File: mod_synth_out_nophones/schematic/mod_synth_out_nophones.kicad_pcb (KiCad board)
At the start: 2 copper layers, 81.9 x 109.2 mm, 50 parts, among them J1 L IN, J2 R IN, J3 Conn_02x08_Odd_Even, J5 L OUT, J6 R OUT, J7 Conn_01x07_Female, J8 Conn_01x07_Male, Q1 2N3904, Q2 2N3904, U1 TL072, U2 TL072

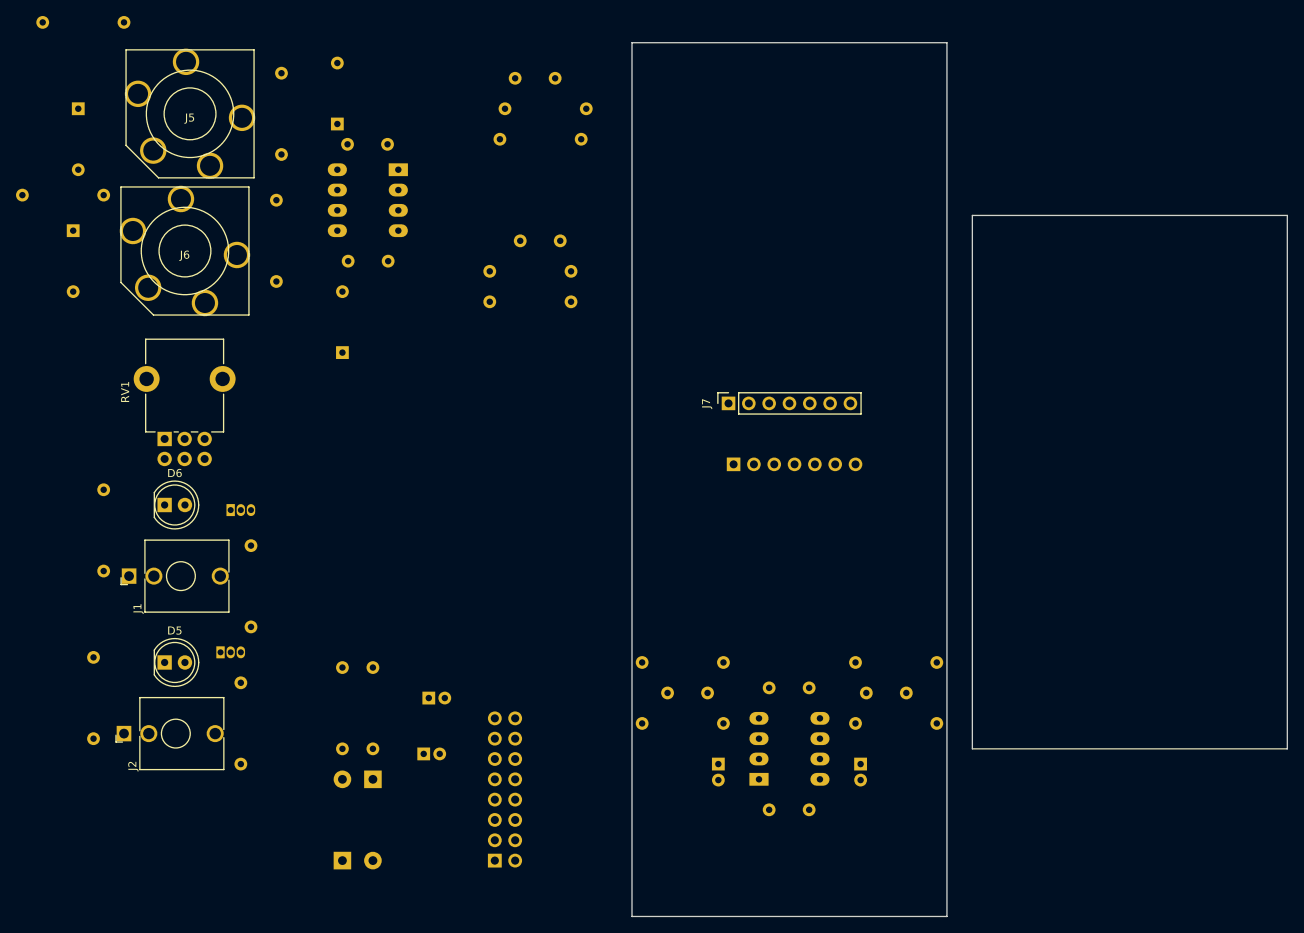
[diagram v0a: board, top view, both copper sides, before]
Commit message: Layout components
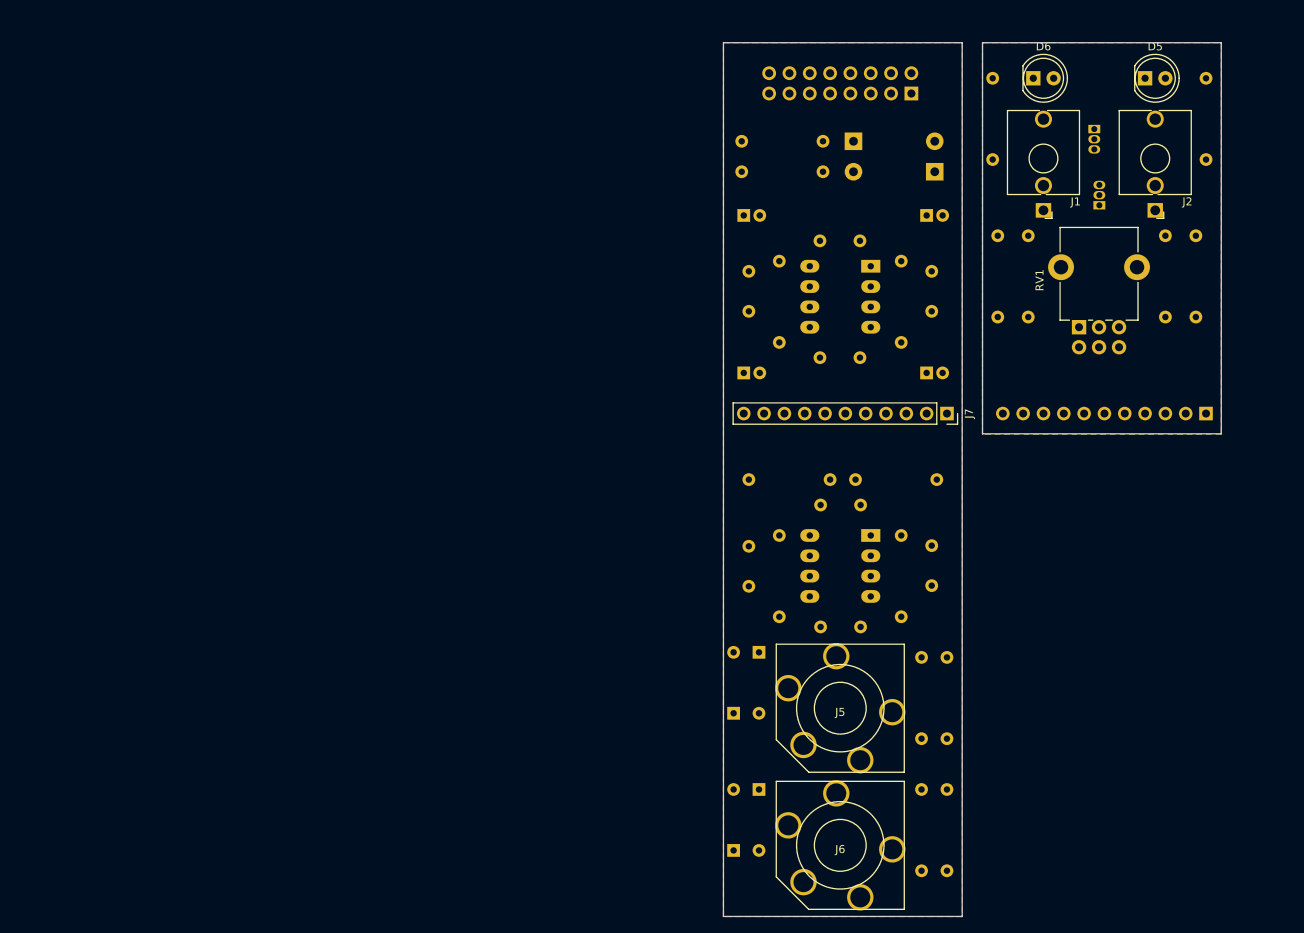
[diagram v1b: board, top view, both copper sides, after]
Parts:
- J7: value Conn_01x07_Female -> Conn_01x11_Female; footprint Connector_PinSocket_2.54mm:PinSocket_1x07_P2.54mm_Vertical -> Connector_PinSocket_2.54mm:PinSocket_1x11_P2.54mm_Vertical
- J8: value Conn_01x07_Male -> Conn_01x011_Male; footprint Connector_PinHeader_2.54mm:PinHeader_1x07_P2.54mm_Vertical -> Connector_PinHeader_2.54mm:PinHeader_1x11_P2.54mm_Vertical
- moved R23 156.8 mm to (266.7, 48.9)
- moved J2 144.5 mm to (260.4, 55.2), turned to 180 degrees
- moved D5 142.7 mm to (259.1, 38.7)
- moved R21 127.8 mm to (265.4, 68.6), turned to 90 degrees
- moved R17 127.4 mm to (231.1, 111.1), turned to 270 degrees
- moved R18 126.4 mm to (231.1, 127.6), turned to 270 degrees
- moved Q1 123.3 mm to (253.4, 54.6), turned to 90 degrees
- moved J1 123.1 mm to (246.4, 55.2), turned to 180 degrees
- moved R24 122.5 mm to (240.0, 48.9)
- moved D6 121.0 mm to (245.1, 38.7)
- moved R20 118.5 mm to (234.3, 137.8), turned to 90 degrees
- moved Q2 118.0 mm to (252.7, 45.1), turned to 270 degrees
- moved R19 117.6 mm to (234.3, 121.3), turned to 90 degrees
- moved RV1 115.2 mm to (250.8, 69.8)
- moved D7 113.6 mm to (232.8, 50.4), turned to 180 degrees
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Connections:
- C10 pad 1: /GND_PCB_B -> GND
- C10 pad 2: /+12_PCB_B -> +12V
- C5 pad 2: Net-(C5-Pad2) -> /B_IN_L
- C6 pad 2: Net-(C6-Pad2) -> /B_IN_R
- C7 pad 1: /-12_PCB_B -> -12V
- C7 pad 2: /GND_PCB_B -> GND
- C8 pad 2: Net-(C8-Pad2) -> /B_RAW_ML
- C9 pad 2: Net-(C9-Pad2) -> /B_RAW_MR
- J7 pad 4: Net-(J7-Pad4) -> /B_IN_L
- J7 pad 5: Net-(J7-Pad5) -> /B_IN_R
- J8 pad 4: Net-(J8-Pad4) -> /A_IN_L
- J8 pad 5: Net-(J8-Pad5) -> /A_IN_R
- R1 pad 1: Net-(C5-Pad2) -> /A_IN_L
- R2 pad 1: Net-(C6-Pad2) -> /A_IN_R
- R3 pad 2: Net-(C5-Pad2) -> /B_IN_L
- R4 pad 2: Net-(C6-Pad2) -> /B_IN_R
- RV1 pad 3: Net-(C8-Pad2) -> /A_RAW_ML
- RV1 pad 6: Net-(C9-Pad2) -> /A_RAW_MR
- U1 pad 2: Net-(C5-Pad2) -> /B_IN_L
- U1 pad 4: /-12_PCB_B -> -12V
- U1 pad 6: Net-(C6-Pad2) -> /B_IN_R
- U1 pad 8: /+12_PCB_B -> +12V
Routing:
- added copper zone on F.Cu, net /GND_PCB_B
- added copper zone on F.Cu, net GND
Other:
- board size 81.9 x 109.2 mm -> 62.2 x 109.2 mm
